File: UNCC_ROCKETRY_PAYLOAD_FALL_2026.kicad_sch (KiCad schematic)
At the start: 0 parts

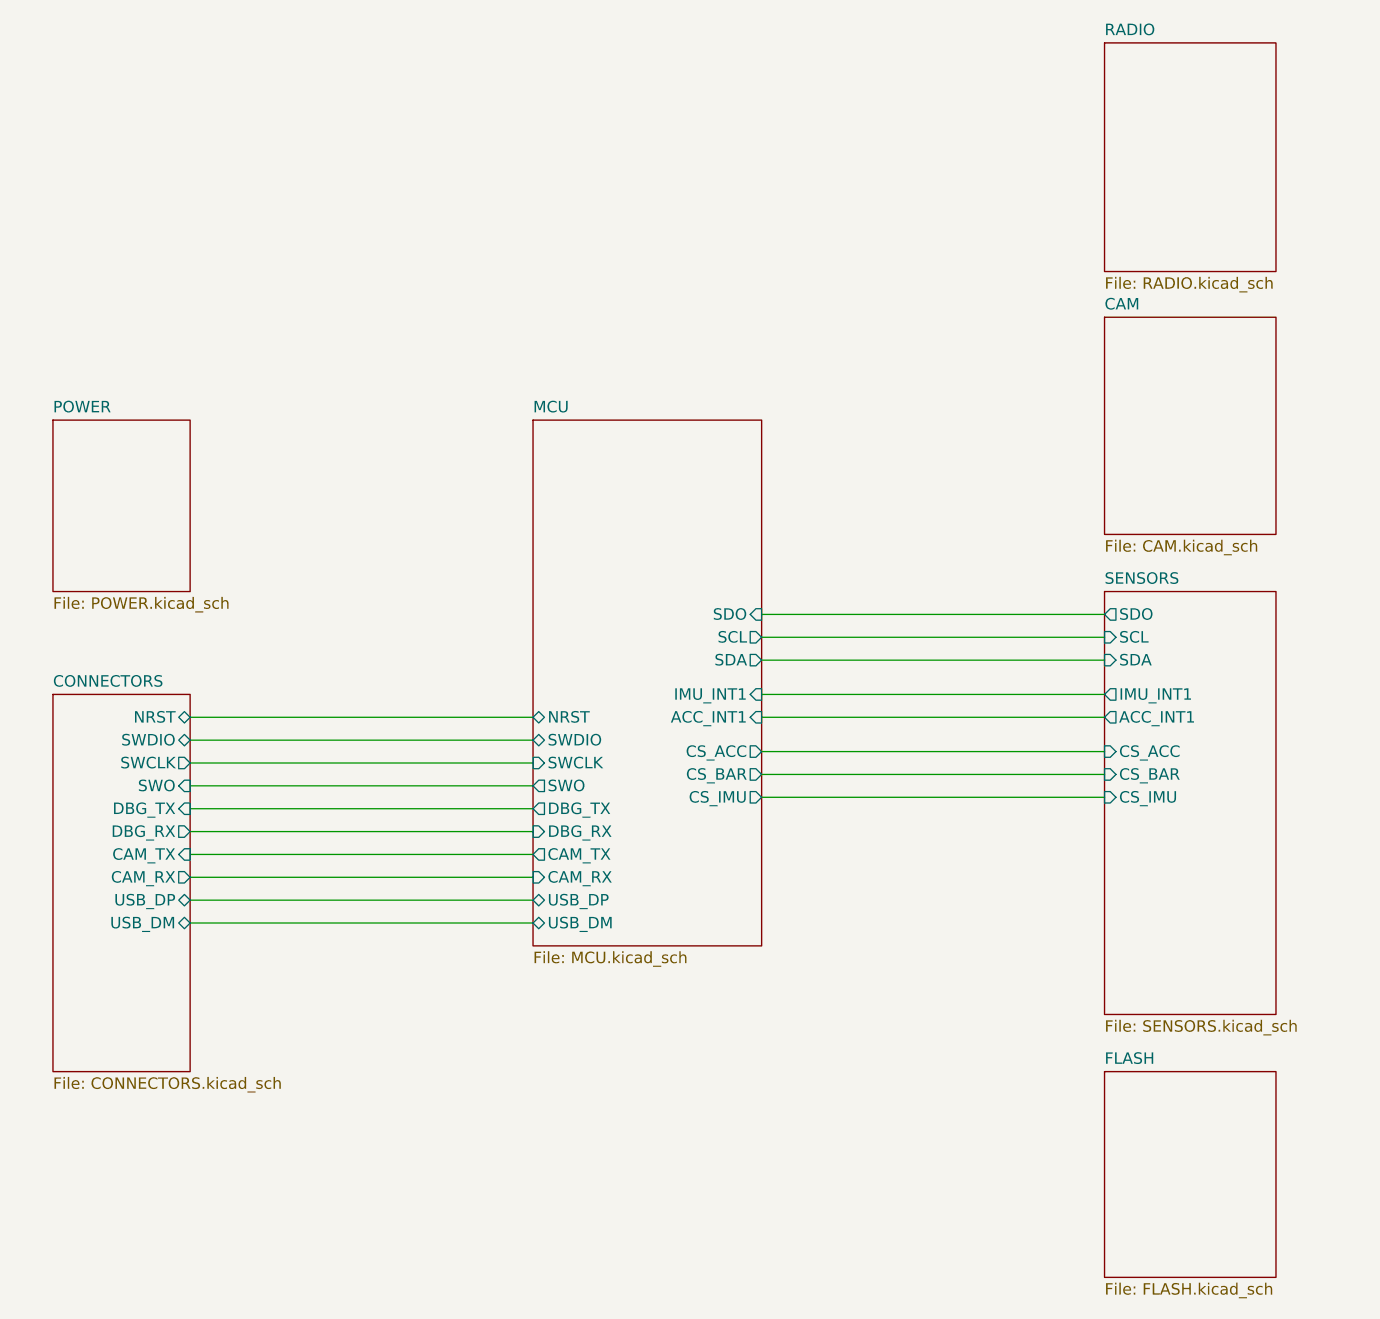
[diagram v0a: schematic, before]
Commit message: cleaned up Schematic
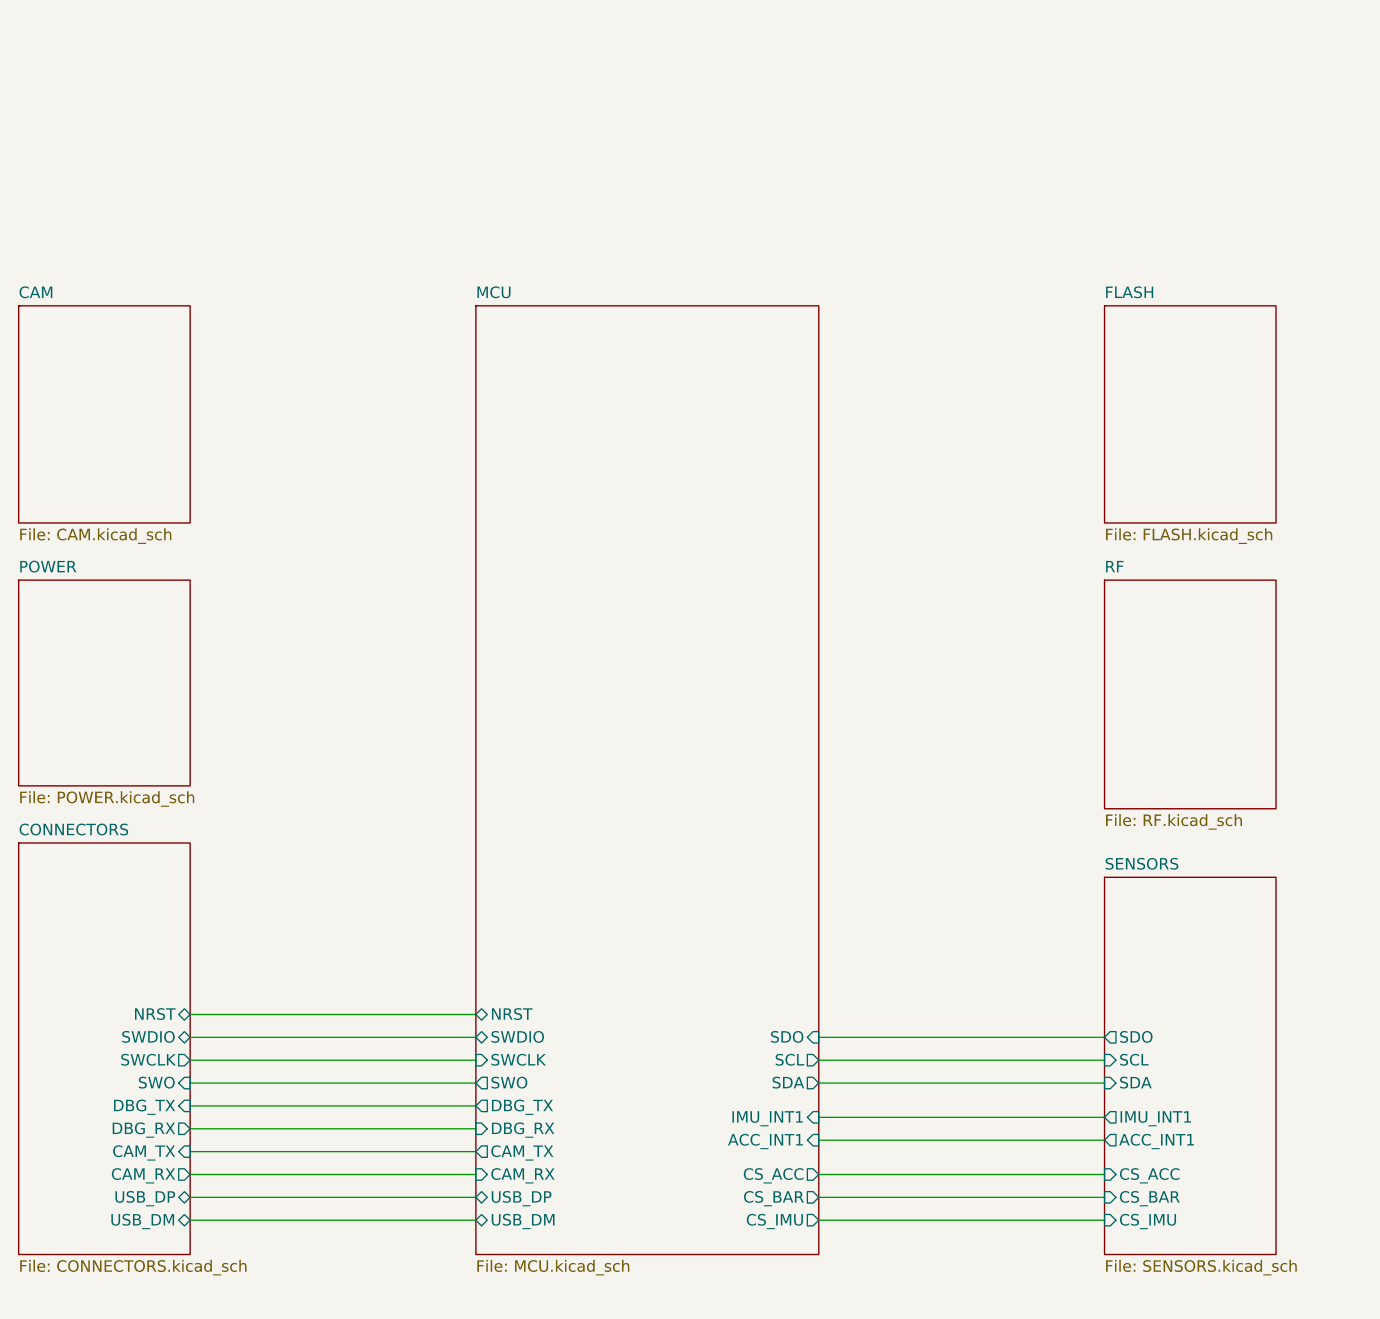
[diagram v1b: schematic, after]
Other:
- sheet RADIO renamed RF
- sheet RF: file RADIO.kicad_sch -> RF.kicad_sch
